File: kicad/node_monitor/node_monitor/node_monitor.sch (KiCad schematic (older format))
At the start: 17 parts, among them J1 Conn_01x02_Male, J2 Conn_01x02_Male, J3 Conn_01x03_Male, J4 RJ45, J5 Conn_01x02_Male, J6 Conn_01x03_Male, J7 Conn_01x03_Male, J8 Conn_01x02_Male, SW1 SW_DIP_x06

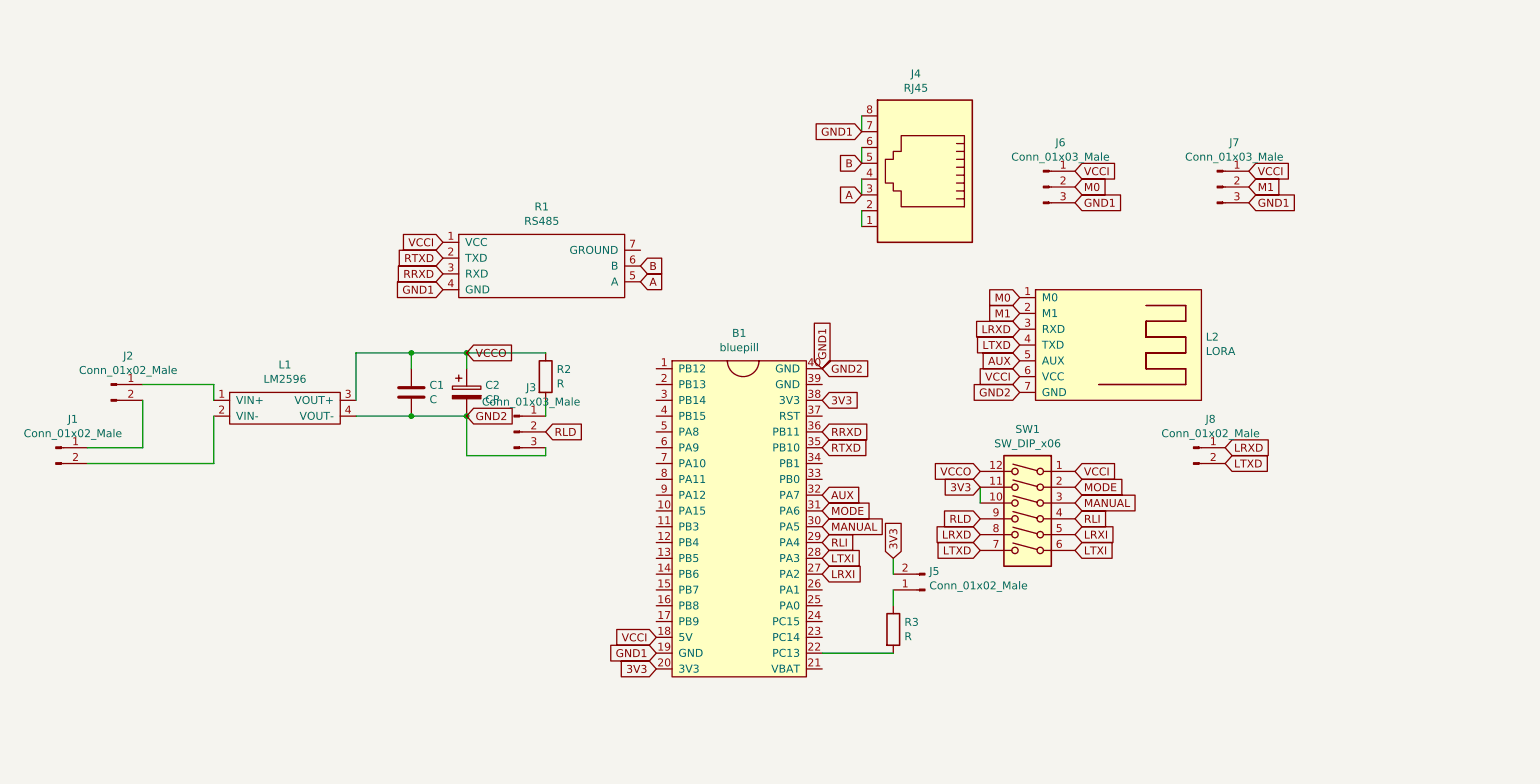
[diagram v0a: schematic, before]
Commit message: 3698
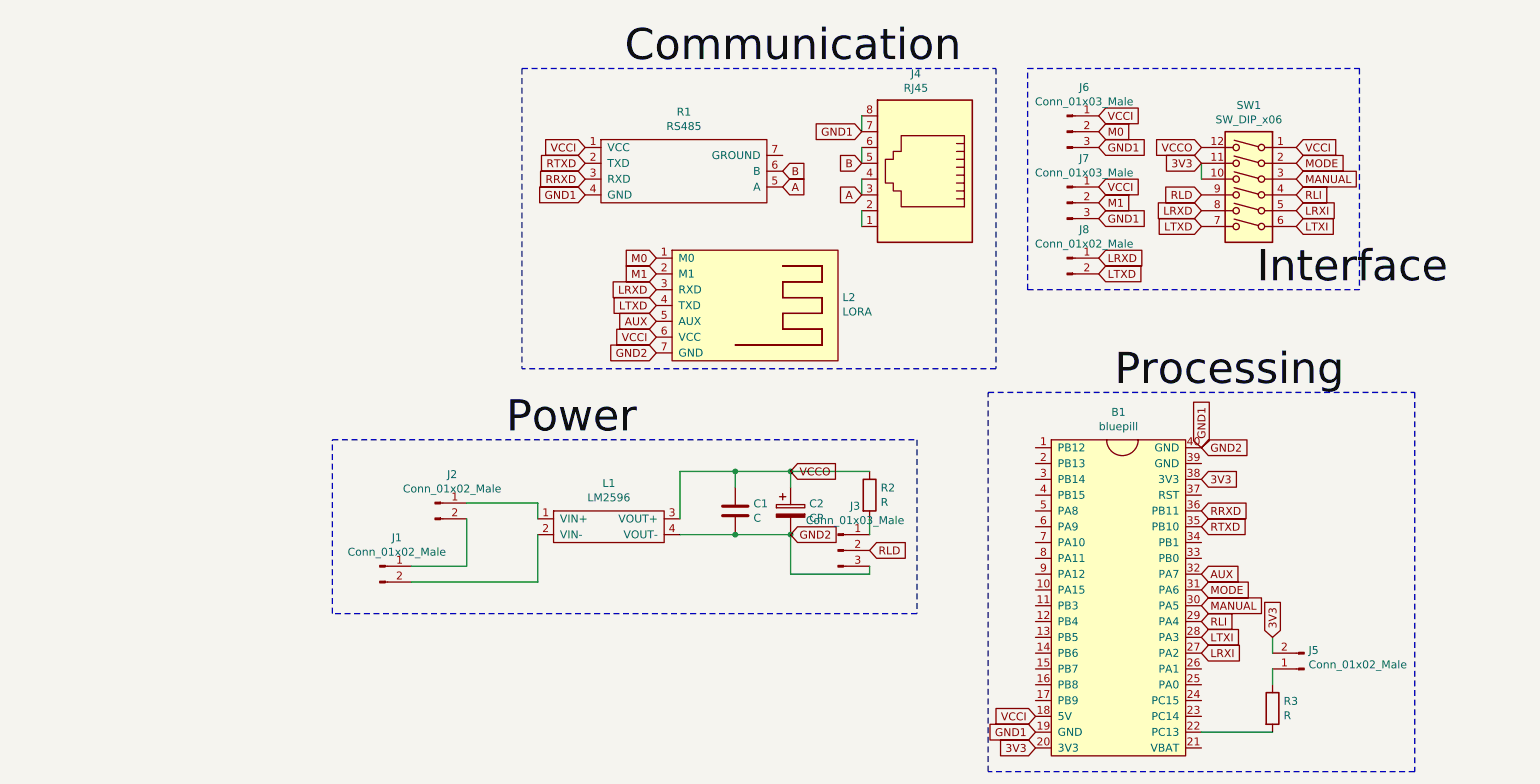
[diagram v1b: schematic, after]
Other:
- moved on the sheet: B1, C1, C2, J1, J2, J3, J5, J6, J7, J8, L1, L2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
